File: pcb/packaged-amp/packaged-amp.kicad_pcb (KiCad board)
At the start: 4 copper layers, 70 x 86 mm, 110 parts, among them J2 RFShield_TwoPieces, J7 Conn_Coaxial, J8 USB_B, Q1 MMBT3906, Q2 MMBT3904, U1 TLV2172, U2 OPA2822, U3 LMR62014XMF, U4 L78L06_SOT89, U5 L79L05_SOT89

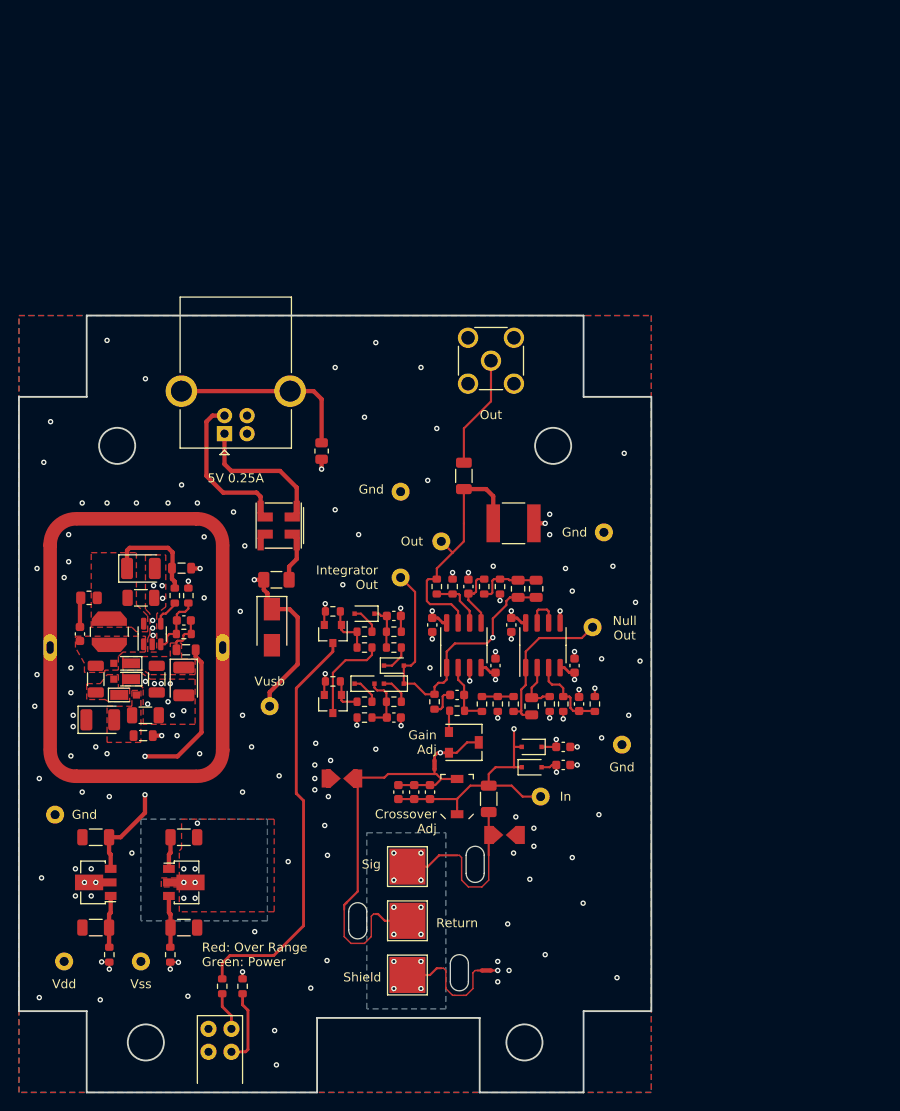
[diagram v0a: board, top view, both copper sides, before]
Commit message: next design revision
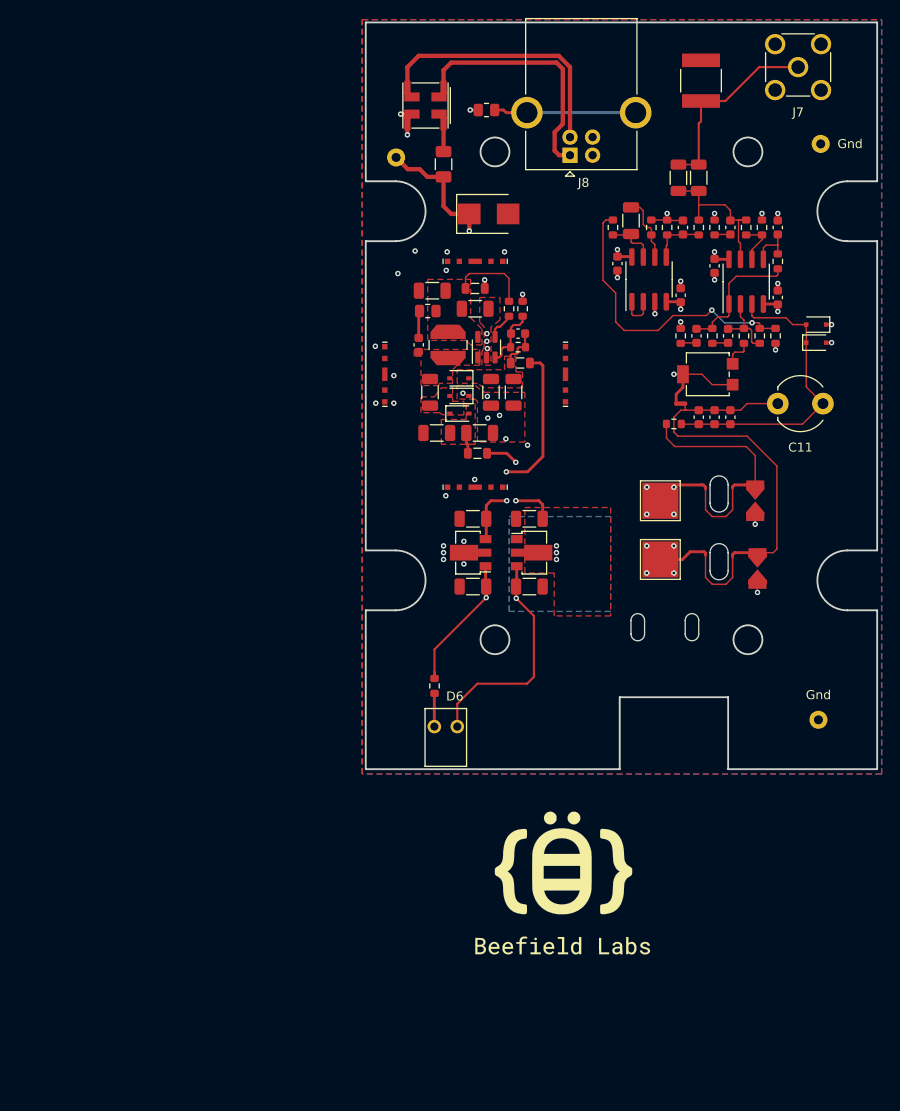
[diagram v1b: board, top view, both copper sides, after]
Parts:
- removed C18: 47n, Capacitor_SMD:C_0805_2012Metric
- removed C24, C26, C32: 47u, Capacitor_Tantalum_SMD:CP_EIA-3528-15_AVX-H
- removed C33, C34: C, Capacitor_SMD:C_0603_1608Metric
- removed C8: 0.47u, Capacitor_SMD:C_0603_1608Metric
- removed D10: LED_Dual_KAKA, wbraun_smd:LED_WP934MD
- removed D7: 1N4148, Diode_SMD:D_SOD-323F
- removed D8, D9: MM3Z7V5B, Diode_SMD:D_SOD-323F
- removed NT2: NetTie_2, NetTie:NetTie-2_SMD_Pad0.5mm
- removed Q1: MMBT3906, wbraun_smd:SOT-23
- removed Q2: MMBT3904, wbraun_smd:SOT-23
- removed R22, R23, R27: 47k, Resistor_SMD:R_0603_1608Metric
- removed R24, R29: 22k, Resistor_SMD:R_0603_1608Metric
- removed R26: 1M, Resistor_SMD:R_0603_1608Metric
- removed R28, R30: 4.7k, Resistor_SMD:R_0603_1608Metric
- removed R31, R32: 0, Resistor_SMD:R_0603_1608Metric
- removed TP1, TP10, TP2, TP3, TP5, TP7, TP8, TP9: TestPoint, wbraun_smd:THM_MINI
- removed TP13: TestPoint, TestPoint:TestPoint_Pad_4.0x4.0mm
- added C2: 10u, Capacitor_SMD:C_1206_3216Metric, F.Cu at (92.2, 105.0)
- added C3: 10u, Capacitor_SMD:C_1206_3216Metric, F.Cu at (83.8, 109.5)
- added C4: DNP, Capacitor_SMD:C_0603_1608Metric, F.Cu at (112.5, 98.8)
- added G***: LOGO, wbraun_smd:Beefield_logo, F.Cu at (97.8, 159.2)
- added J1: ECT81800C036, wbraun_smd:Shield_Clip_ECT81800C036, F.Cu at (88.0, 90.5)
- added J3: ECT81800C036, wbraun_smd:Shield_Clip_ECT81800C036, F.Cu at (88.0, 115.5)
- added J4: ECT81800C036, wbraun_smd:Shield_Clip_ECT81800C036, F.Cu at (98.0, 103.0)
- C10: value 22p -> DNP
- C11: value 8-40p -> 12-60p; footprint Capacitor_SMD:C_Trimmer_Voltronics_JZ -> wbraun_smd:C_Trimmer_GKG_6mm
- C15: footprint Capacitor_SMD:C_0805_2012Metric -> Capacitor_SMD:C_1206_3216Metric
- C17: value 47n -> DNP; footprint Capacitor_SMD:C_0805_2012Metric -> Capacitor_SMD:C_0603_1608Metric
- C19: value 22p -> 10p
- C22: value 470p -> 330p
- C7: value 0.47u -> 10u; footprint Capacitor_SMD:C_0603_1608Metric -> Capacitor_SMD:C_1206_3216Metric
- C9: value 150p -> 100p
- D11: value SMAJ6.0A-13-F -> P6SMB6.8CA/TR13; footprint Diode_SMD:D_SMA -> Diode_SMD:D_SMB
- D3, D4, D5: value PD3S140-7 -> BAT760-7; footprint wbraun_smd:D_POWERDI323 -> Diode_SMD:D_SOD-323
- D6: value 1N4148 -> LTST-S220KGKT; footprint Diode_SMD:D_SOD-323F -> wbraun_smd:LED-T1-RIGHT-ANGLE_4.6x4.4mm
- J2: value RFShield_TwoPieces -> ECT81800C036; footprint wbraun_smd:Masach_Tech_MS288-10F -> wbraun_smd:Shield_Clip_ECT81800C036
- L2: value L_Ferrite_Coupled -> DLW5BTM142SQ2L
- R1: footprint Resistor_SMD:R_1206_3216Metric -> Resistor_SMD:R_0603_1608Metric
- R10: value 220 -> 470
- R11, R12: value 2k -> 470
- R13: value 47 -> 100
- R15, R18: value 75k -> 82k
- R16: value 13.3k -> 13k
- R19: value R -> DNP
- R2: value 4.7k -> 22k
- R20: value 2k -> DNP
- R21: value 2k -> 100; footprint Resistor_SMD:R_0603_1608Metric -> Resistor_SMD:R_1206_3216Metric
- R25: value 1M -> 4.7k
- R3: value 10k -> 8.2k
- R4, R7: value 47k -> 22k
- R6: value 22k -> DNP
- R8: value 2k -> 10k
- R9: value 10k -> 2k
- RV1: footprint wbraun_smd:TRIMMER_PVG3A -> Potentiometer_SMD:Potentiometer_Bourns_3314G_Vertical
- U4: value L78L06_SOT89 -> MC78L06F-TP
- U5: value L79L05_SOT89 -> MC79L06F-TP
- moved TP4 112.7 mm to (126.2, 77.5)
- moved R20 63.4 mm to (114.5, 86.8), turned to 90 degrees
- moved TP14 62.3 mm to (79.2, 79.0)
- moved R21 60.8 mm to (110.5, 81.2), turned to -90 degrees
- moved C11 57.8 mm to (124.0, 106.2), turned to 180 degrees
- moved D2 56.6 mm to (125.8, 99.5)
- moved D1 56.4 mm to (125.8, 97.5)
- moved C30 56.3 mm to (87.8, 126.5)
- moved U4 55.3 mm to (87.5, 122.8)
- moved C15 54.9 mm to (105.2, 86.0)
- moved C28 54.6 mm to (87.8, 119.0)
- moved C16 54.0 mm to (111.0, 86.8), turned to -90 degrees
- moved R8 54.0 mm to (112.8, 86.8), turned to 90 degrees
- moved R4 53.9 mm to (103.2, 86.8)
- moved C31 53.7 mm to (94.0, 126.5)
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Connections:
- net Net-(C14-Pad1) renamed /int_fb
- C16 pad 1: Net-(C16-Pad1) -> GND
- C16 pad 2: GND -> Net-(C16-Pad2)
- C17 pad 1: /int_out -> /out
- C30 pad 1: Net-(C30-Pad1) -> VDD
- C31 pad 2: Net-(C31-Pad2) -> VSS
- C7 pad 1: GND -> /VBUS
- C7 pad 2: VDD -> GND
- D6 pad 1: /int_out -> VSS
- J7 pad 1: Net-(J7-Pad1) -> Net-(GD1-Pad1)
- R10 pad 2: Net-(C17-Pad2) -> /int_out
- R12 pad 1: Net-(GD1-Pad1) -> /out
- R13 pad 1: Net-(J7-Pad1) -> Net-(GD1-Pad1)
- R13 pad 2: Net-(GD1-Pad1) -> /out
- R20 pad 1: Net-(D6-Pad2) -> Net-(C17-Pad2)
- R20 pad 2: Net-(C33-Pad1) -> GND
- R21 pad 1: Net-(D7-Pad1) -> Net-(GD1-Pad1)
- R21 pad 2: Net-(C34-Pad1) -> /out
- R25 pad 1: Net-(Q1-Pad1) -> Net-(D6-Pad2)
- R6 pad 1: Net-(C15-Pad2) -> Net-(C4-Pad2)
- R7 pad 1: Net-(C16-Pad1) -> Net-(C15-Pad2)
- R7 pad 2: /int_out -> GND
- R8 pad 1: GND -> Net-(C16-Pad2)
- R8 pad 2: Net-(C16-Pad1) -> /out
- R9 pad 2: Net-(C17-Pad2) -> Net-(C16-Pad2)
- RV1 pad 1: Net-(R5-Pad1) -> GND
- RV1 pad 3: GND -> Net-(R5-Pad1)
- U1 pad 1: Net-(C15-Pad1) -> Net-(U1-Pad1)
- U1 pad 2: Net-(C15-Pad2) -> Net-(U1-Pad1)
- U1 pad 3: Net-(C16-Pad1) -> GND
- U1 pad 5: GND -> Net-(C16-Pad2)
- U1 pad 6: Net-(U1-Pad6) -> Net-(C15-Pad2)
- U1 pad 7: Net-(U1-Pad6) -> Net-(C15-Pad1)
- U2 pad 7: Net-(GD1-Pad1) -> /out
- U4 pad 1: Net-(C30-Pad1) -> VDD
- U5 pad 3: Net-(C31-Pad2) -> VSS
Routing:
- net Net-(Q2-Pad3): track 45.8 -> 0.00 mm
- net /int_out: track 49.8 -> 14.6 mm, vias 2 -> 0
- net Net-(R2-Pad2): track 3.50 -> 33.0 mm, vias 0 -> 2
- net /out: track 0.00 -> 16.8 mm
- net VSS: track 15.2 -> 30.7 mm, vias 8 -> 4
- net Net-(NT2-Pad1): track 13.1 -> 0.00 mm, vias 4 -> 0
- net Net-(E1-Pad2): track 20.3 -> 33.1 mm
- net Net-(J8-Pad4): track 16.4 -> 29.0 mm
- net Net-(J7-Pad1): track 12.5 -> 0.00 mm
- net Net-(J8-Pad1): track 14.6 -> 27.0 mm
- net Net-(C15-Pad1): track 17.7 -> 5.74 mm
- net Net-(Q1-Pad3): track 10.4 -> 0.00 mm
- net /return_kelvin: track 45.7 -> 56.1 mm
- net Net-(C16-Pad1): track 9.22 -> 0.00 mm
- net Net-(D10-Pad3): track 8.36 -> 0.00 mm
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- added copper zone on B.Cu, net GND
- added copper zone on In2.Cu, net GND
- added copper zone on In2.Cu, net VDD
- removed copper zone on B.Cu, net VDD
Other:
- board size 70 x 86 mm -> 56.6 x 82.7 mm
- board text removed: "5V 0.25A"
- board text removed: "Crossover Adj"
- board text removed: "Designed to fit hammond 1593BBBK enclosure"
- board text removed: "Gain Adj"
- board text removed: "In"
- board text removed: "Integrator Out"
- board text removed: "Null Out"
- board text removed: "Out"
- board text removed: "Red: Over Range Green: Power"
- board text removed: "Return"
- board text removed: "Shield"
- board text removed: "Sig"
- board text removed: "Vdd"
- board text removed: "Vss"
- board text removed: "Vusb"
